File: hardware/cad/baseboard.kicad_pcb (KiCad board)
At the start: 6 copper layers, 102.3 x 60 mm, 111 parts, among them J201 ACJS-IHS, J202 SFV20R-2STE1HLF, J203 ACJS-IHS, J301 PJ-063AH, J401 6-440054-2, J403 2x2 PIN HEADER, J404 6-440054-2, J406 6-440054-2, J408 6-440054-2, Q401 DMN2050, Q402 DMN2050, U201 ADG5434, U301 LM337KVURG3, U302 LM317MDT-TR, U303 ADP5070, U304 LM317MDT-TR, U401 STM32G031K8U6

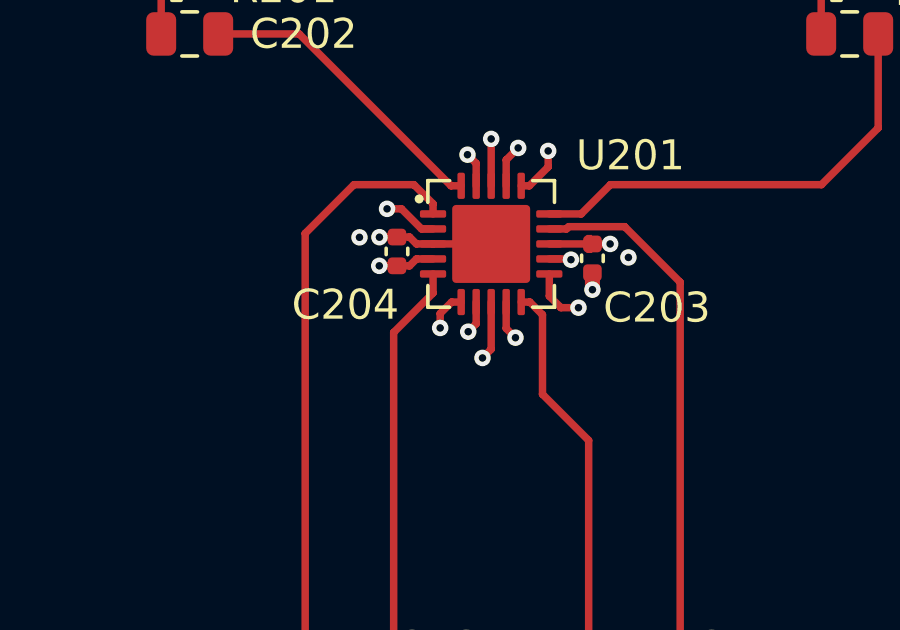
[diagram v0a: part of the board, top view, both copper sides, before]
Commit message: finalization before first board spin
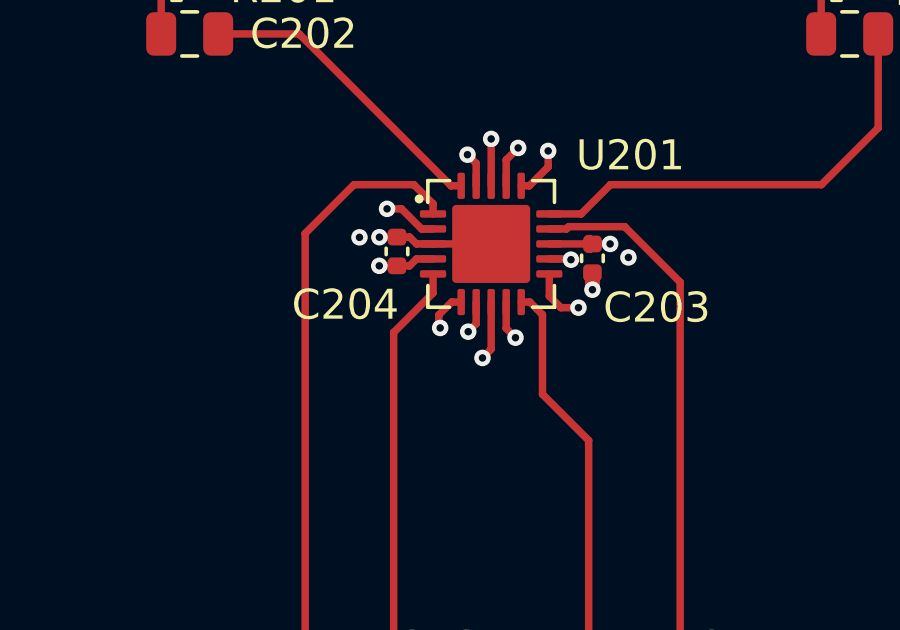
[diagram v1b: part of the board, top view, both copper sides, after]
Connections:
- G201 pad 1: (no net) -> GND
- G202 pad 1: (no net) -> GND
- G301 pad 1: (no net) -> GND
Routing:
- added copper zone on In4.Cu, net GND
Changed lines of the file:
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@@
     (grid_origin 41.5 133.3)
     (pcbplotparams
-      (layerselection 0x00302fc_ffffffff)
+      (layerselection 0x00000fc_ffffffff)
       (plot_on_all_layers_selection 0x0001000_00000000)
       (disableapertmacros false)
@@
       (sketchpadsonfab false)
       (subtractmaskfromsilk false)
-      (outputformat 4)
+      (outputformat 1)
       (mirror false)
-      (drillshape 2)
+      (drillshape 0)
       (scaleselection 1)
       (outputdirectory "gerbers")
@@
     (property "ki_description" "Power symbol creates a global label with name \"Chassis\" , chassis ground")
     (property "ki_keywords" "power-flag")
+    (zone_connect 1)
     (attr smd)
     (fp_text reference "G202" (at 0 -4.5 unlocked) (layer "B.SilkS")
@@
     (fp_rect (start -1.7 3.9) (end 1.7 -3.9)
       (stroke (width 0.05) (type solid)) (fill none) (layer "B.CrtYd"))
-    (pad "1" smd roundrect (at 0 0 180) (size 3 7.5) (layers "B.Cu" "B.Paste" "B.Mask") (roundrect_rratio 0.1))
+    (pad "1" smd roundrect (at 0 0 180) (size 3 7.5) (layers "B.Cu" "B.Paste" "B.Mask") (roundrect_rratio 0.1)
+      (net 69 "GND"))
     (model "${KIPRJMOD}/packages3D/s7061-46r.stp"
       (offset (xyz 0 -3.5 0))
@@
     (property "ki_description" "Power symbol creates a global label with name \"Chassis\" , chassis ground")
     (property "ki_keywords" "power-flag")
+    (zone_connect 1)
     (attr smd)
     (fp_text reference "G201" (at 0 -4.5 unlocked) (layer "B.SilkS")
@@
     (fp_rect (start -1.7 3.9) (end 1.7 -3.9)
       (stroke (width 0.05) (type solid)) (fill none) (layer "B.CrtYd"))
-    (pad "1" smd roundrect (at 0 0 180) (size 3 7.5) (layers "B.Cu" "B.Paste" "B.Mask") (roundrect_rratio 0.1))
+    (pad "1" smd roundrect (at 0 0 180) (size 3 7.5) (layers "B.Cu" "B.Paste" "B.Mask") (roundrect_rratio 0.1)
+      (net 69 "GND"))
     (model "${KIPRJMOD}/packages3D/s7061-46r.stp"
       (offset (xyz 0 -3.5 0))
@@
     (property "ki_description" "Power symbol creates a global label with name \"Chassis\" , chassis ground")
     (property "ki_keywords" "power-flag")
+    (zone_connect 1)
     (attr smd)
     (fp_text reference "G301" (at 0 -4.5 unlocked) (layer "B.SilkS")
@@
     (fp_rect (start -1.7 3.9) (end 1.7 -3.9)
       (stroke (width 0.05) (type solid)) (fill none) (layer "B.CrtYd"))
-    (pad "1" smd roundrect (at 0 0 180) (size 3 7.5) (layers "B.Cu" "B.Paste" "B.Mask") (roundrect_rratio 0.1))
+    (pad "1" smd roundrect (at 0 0 180) (size 3 7.5) (layers "B.Cu" "B.Paste" "B.Mask") (roundrect_rratio 0.1)
+      (net 69 "GND"))
     (model "${KIPRJMOD}/packages3D/s7061-46r.stp"
       (offset (xyz 0 -3.5 0))
@@
   (gr_line (start 251.22 127.77) (end 251.92 127.77)
     (stroke (width 0.1) (type default)) (layer "F.SilkS"))
-  (gr_line (start 202.97 134.67) (end 203.22 134.67)
-    (stroke (width 0.1) (type default)) (layer "Dwgs.User"))
-  (gr_line (start 202.97 135.67) (end 203.22 135.67)
-    (stroke (width 0.1) (type default)) (layer "Dwgs.User"))
-  (gr_line (start 202.97 138.67) (end 203.22 138.67)
-    (stroke (width 0.1) (type default)) (layer "Dwgs.User"))
-  (gr_line (start 202.97 136.67) (end 203.22 136.67)
-    (stroke (width 0.1) (type default)) (layer "Dwgs.User"))
-  (gr_line (start 202.97 133.67) (end 203.22 133.67)
-    (stroke (width 0.1) (type default)) (layer "Dwgs.User"))
-  (gr_line (start 202.97 137.67) (end 203.22 137.67)
-    (stroke (width 0.1) (type default)) (layer "Dwgs.User"))
   (gr_line (start 16.75 255.088) (end 144.26429 255.088)
     (stroke (width 0.1) (type default)) (layer "Cmts.User"))
@@
   (segment (start 228.894999 117.3525) (end 228.895 121.277234) (width 0.25) (layer "F.Cu") (net 44))
   (segment (start 228.895 121.277234) (end 229.68031 122.062544) (width 0.25) (layer "F.Cu") (net 44))
-  (segment (start 195.4025 141.6075) (end 195.72 141.6075) (width 0.25) (layer "F.Cu") (net 45))
   (segment (start 199.045 141.795) (end 199.63 141.795) (width 0.25) (layer "F.Cu") (net 45))
-  (segment (start 195.02 141.99) (end 195.4025 141.6075) (width 0.25) (layer "F.Cu") (net 45))
+  (segment (start 194.975 142.425) (end 195.02 142.47) (width 0.25) (layer "F.Cu") (net 45))
   (segment (start 198.6575 141.4075) (end 199.045 141.795) (width 0.25) (layer "F.Cu") (net 45))
-  (segment (start 195.02 142.47) (end 195.02 141.99) (width 0.25) (layer "F.Cu") (net 45))
+  (segment (start 195.4025 141.6075) (end 194.975 142.035) (width 0.25) (layer "F.Cu") (net 45))
   (segment (start 198.6575 140.67) (end 198.6575 141.4075) (width 0.25) (layer "F.Cu") (net 45))
+  (segment (start 194.975 142.035) (end 194.975 142.425) (width 0.25) (layer "F.Cu") (net 45))
+  (segment (start 195.72 141.6075) (end 195.4025 141.6075) (width 0.25) (layer "F.Cu") (net 45))
   (via (at 199.63 141.795) (size 0.55) (drill 0.25) (layers "F.Cu" "B.Cu") (net 45))
   (via (at 195.02 142.47) (size 0.55) (drill 0.25) (layers "F.Cu" "B.Cu") (net 45))
@@
     )
   )
-  (zone (net 69) (net_name "GND") (layers "In1.Cu" "In2.Cu" "In3.Cu" "B.Cu") (hatch edge 1)
+  (zone (net 69) (net_name "GND") (layers "In1.Cu" "In2.Cu" "In3.Cu" "In4.Cu" "B.Cu") (hatch edge 1)
     (connect_pads yes (clearance 0.25))
     (min_thickness 0.15) (filled_areas_thickness no)
